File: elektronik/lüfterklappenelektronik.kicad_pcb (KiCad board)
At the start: 4 copper layers, 80 x 87.6 mm, 115 parts, among them J101 Conn_01x05_Male, J102 Ckmtw_2510S-2P, J103 Conn_LAN_ENC28J60, J104 USB_B_Micro, J106 WJ2EDGVC-5.08-2P, J107 WJ2EDGVC-5.08-2P, J108 WJ2EDGVC-5.08-2P, P101 PWR_BUS_CONN, P103 PressureSensor3, P104 PressureSensor1, P105 PressureSensor2, P109 PWR_BUS_CONN, Q101 IRLR8743TRPBF, Q102 IRLR8743TRPBF, Q103 IRLR8743TRPBF, Q104 Q_NPN_Darlington_BEC, Q105 Q_NPN_Darlington_BEC, SW101 SW_Push, SW102 SW_Push, U101 Gabellichtschranke, U102 Gabellichtschranke, U103 Gabellichtschranke, U105 ESP32-WROOM-32E, U106 AMS1117-3.3, U107 CP2102N-A01-GQFN28

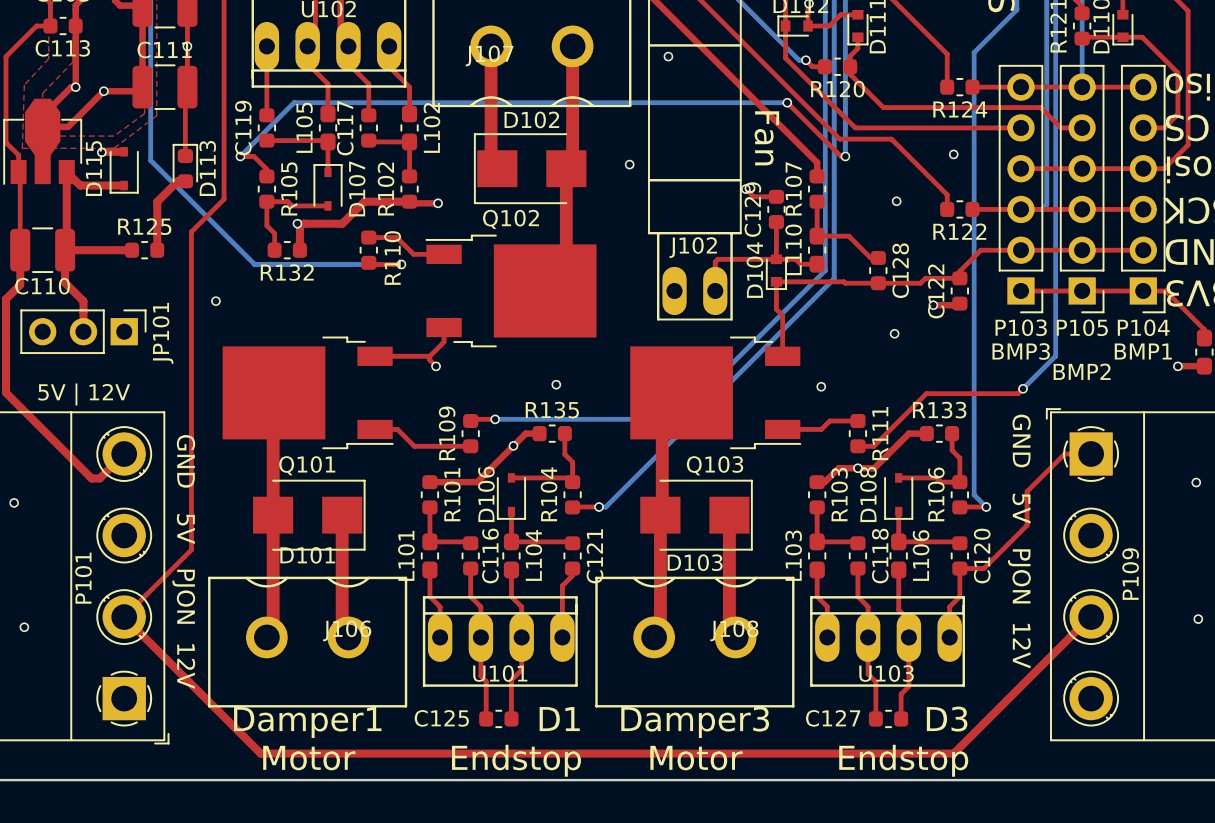
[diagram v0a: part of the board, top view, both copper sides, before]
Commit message: kicad v10 und pdf
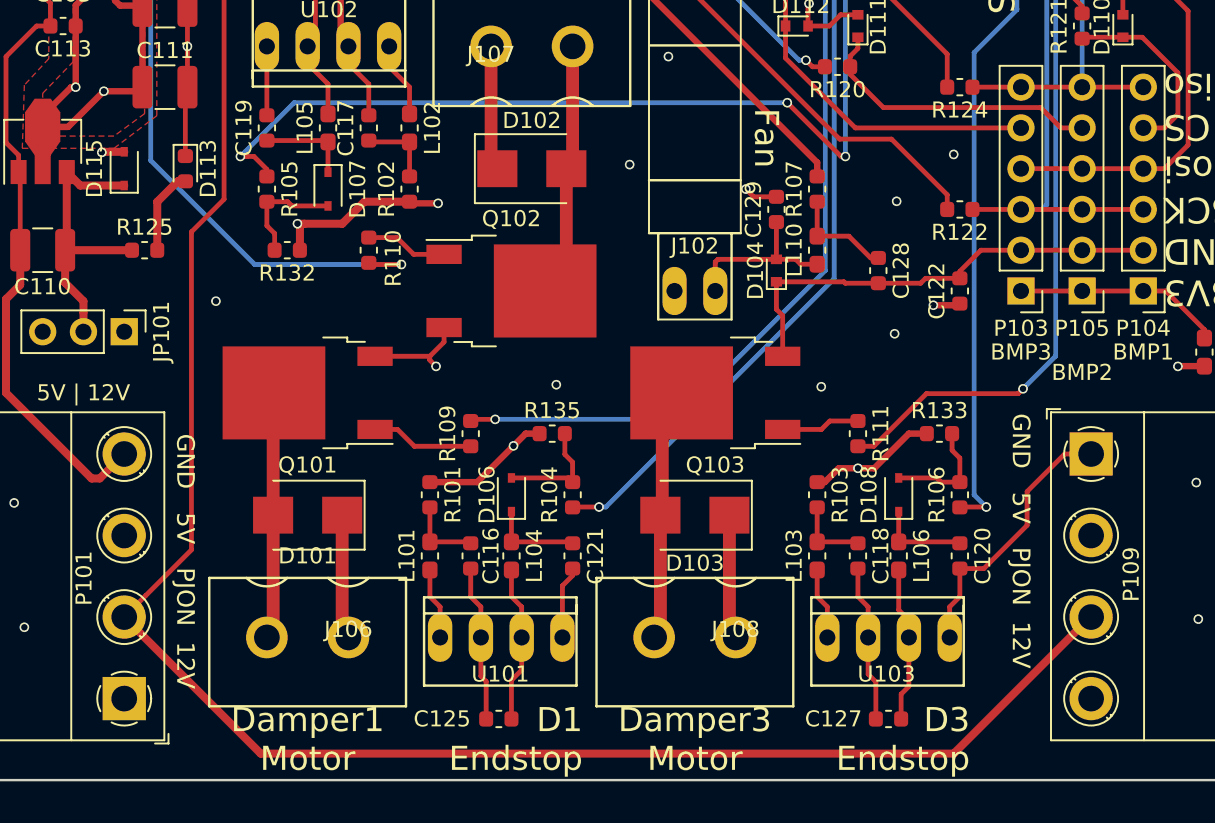
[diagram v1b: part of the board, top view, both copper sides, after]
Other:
- net class 12V removed
- net class 3V3 removed
- net class 5V removed
- net class Default removed
